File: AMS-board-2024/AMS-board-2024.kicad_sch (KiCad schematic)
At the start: 1 part, among them J1 5077CR-16-SMC2-BK-TR

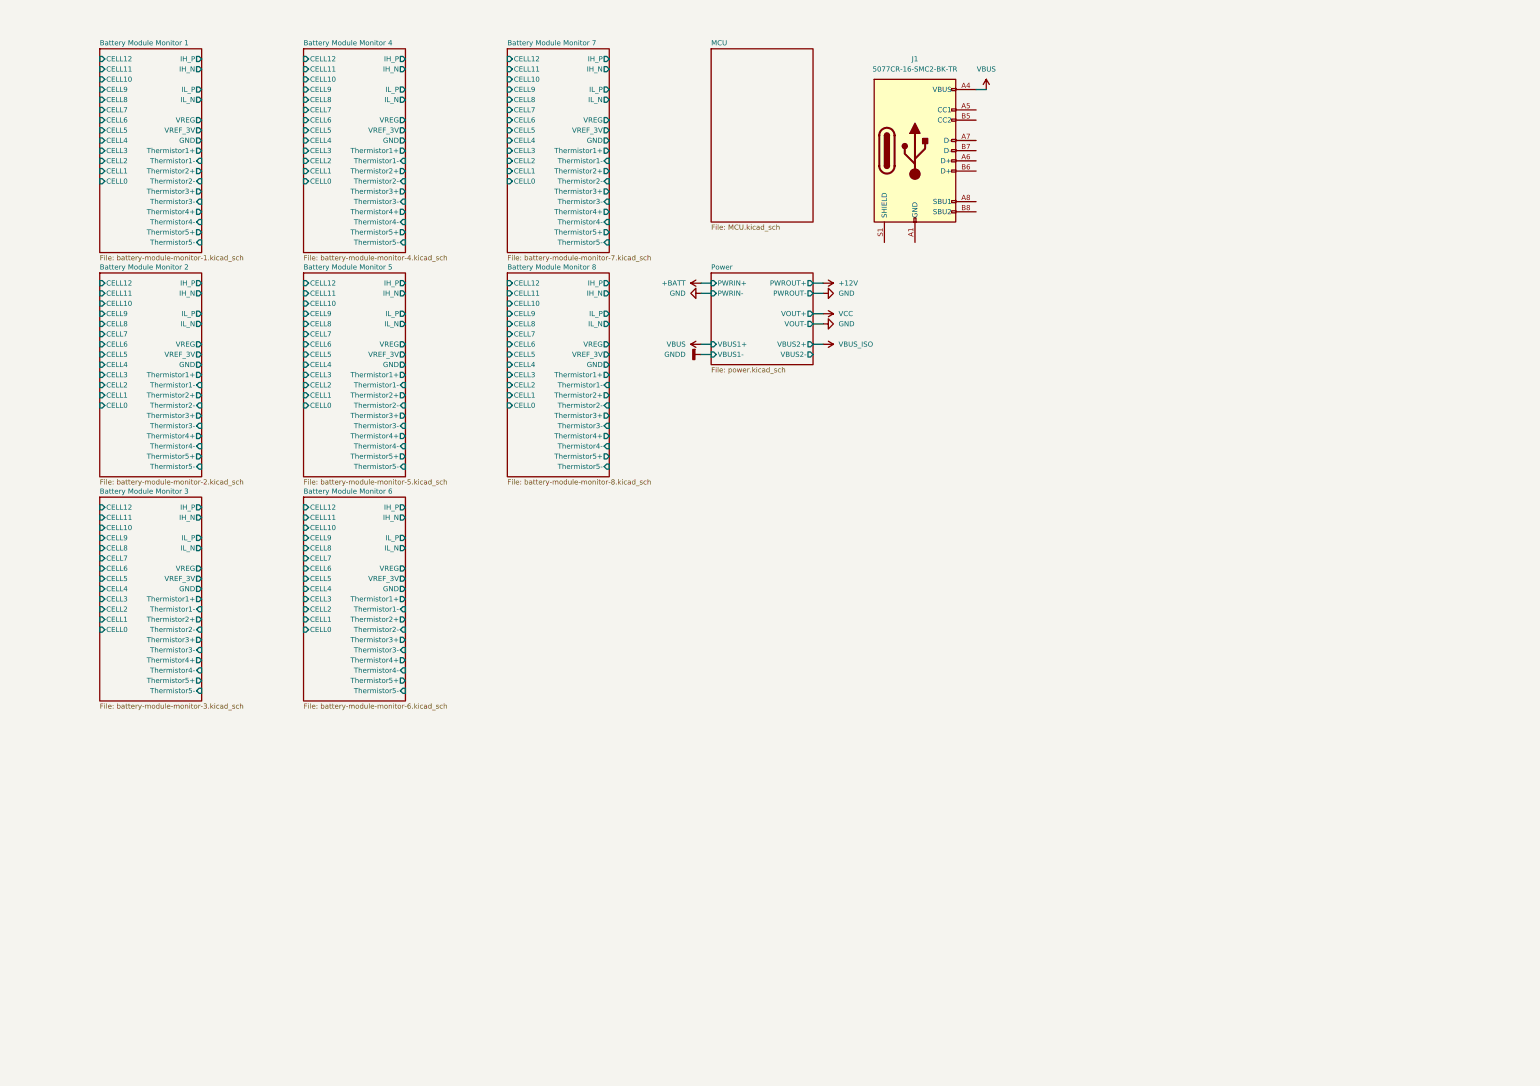
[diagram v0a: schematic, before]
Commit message: アノテーションし直し
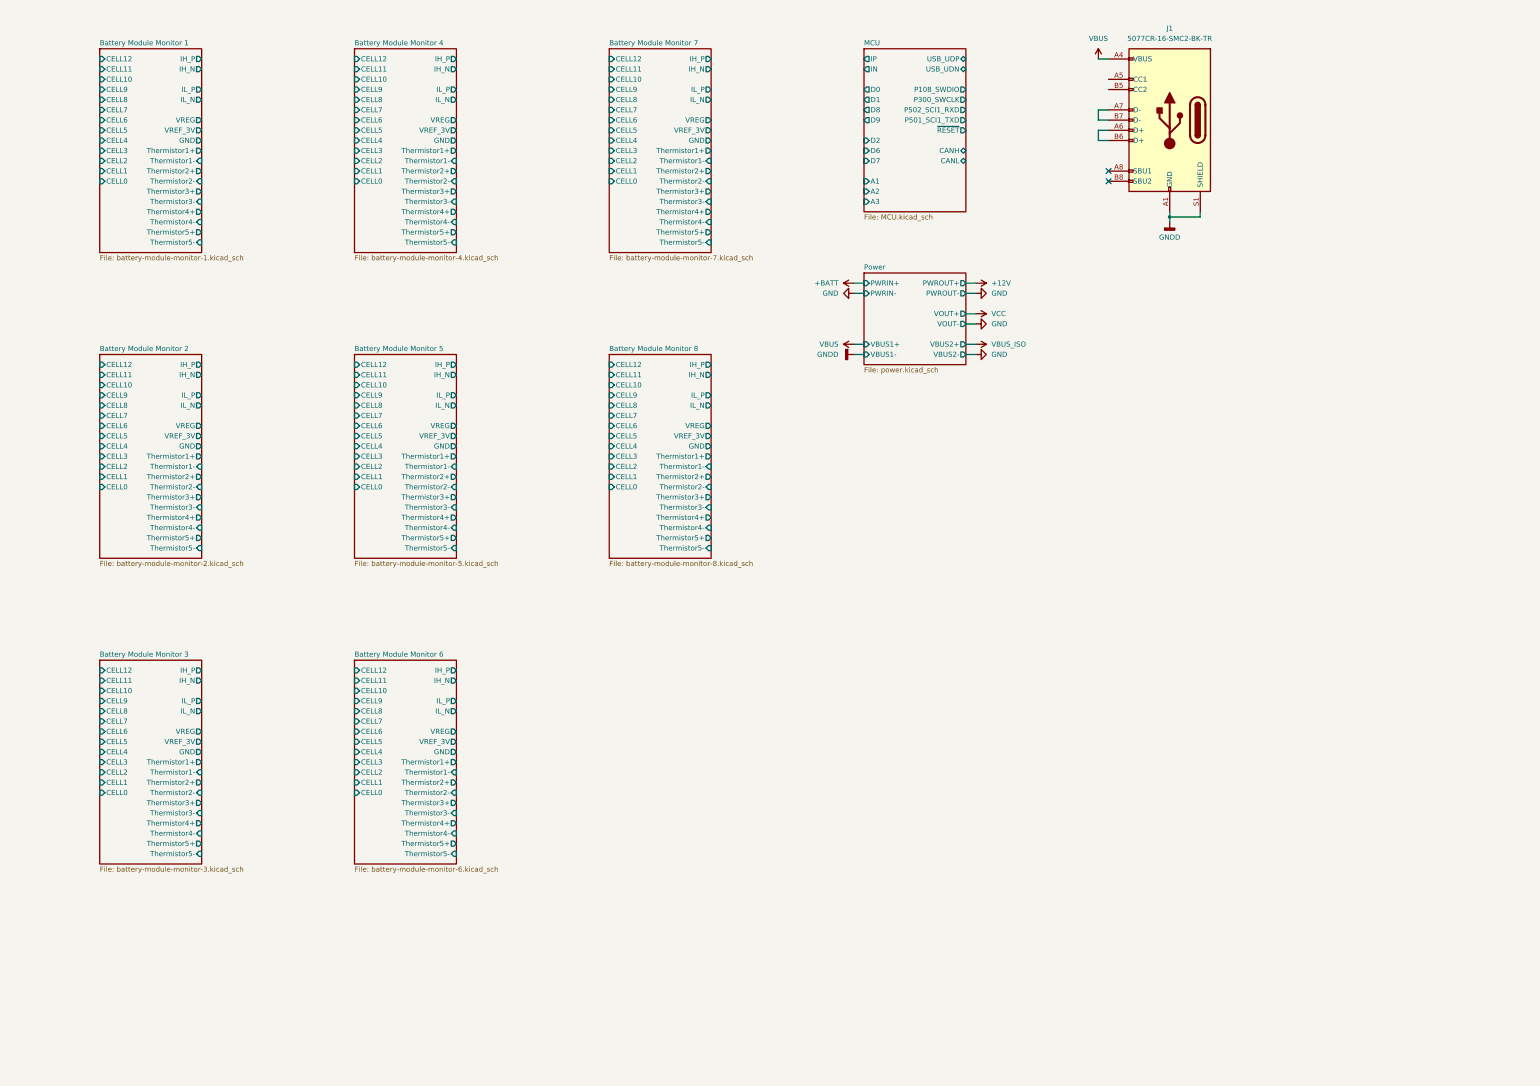
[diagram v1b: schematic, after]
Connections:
- net GNDD: now also J1.A1 (GND), J1.A12 (GND), J1.B1 (GND), J1.B12 (GND), J1.S1 (SHIELD)
- net at J1.A6 (D+): now also J1.B6 (D+)
- net at J1.A7 (D-): now also J1.B7 (D-)
- no-connect marks 0 -> 2
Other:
- sheet MCU ports: added A1, A2, A3, CANH, CANL, D0, D1, D2, D6, D7, D8, D9, IN, IP, P108_SWDIO, P300_SWCLK, P501_SCI1_TXD, P502_SCI1_RXD, USB_UDN, USB_UDP, ~{RESET}; removed none
- moved on the sheet: J1

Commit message: およそ回路図完成
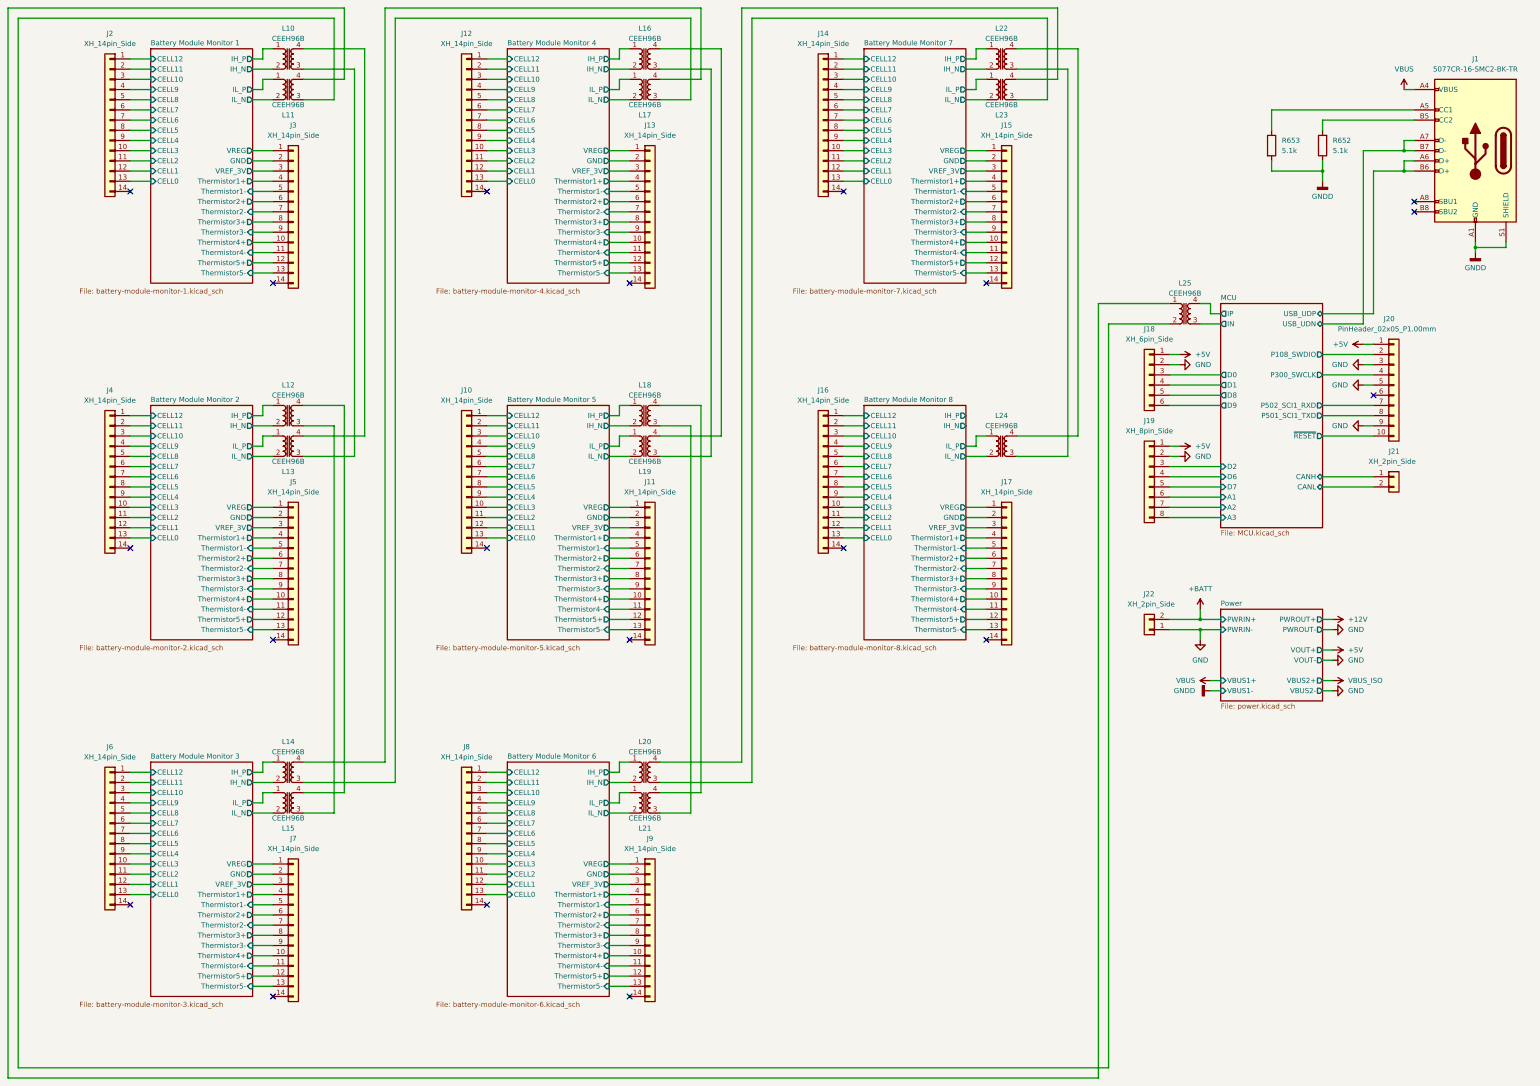
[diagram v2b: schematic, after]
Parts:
- added J10, J11, J12, J13, J14, J15, J16, J17, J2, J3, J4, J5, J6, J7, J8, J9: XH_14pin_Side, Connector_JST:JST_XH_S14B-XH-A_1x14_P2.50mm_Horizontal, symbol Connector_Generic:Conn_01x14
- added J18: XH_6pin_Side, Connector_JST:JST_XH_S6B-XH-A_1x06_P2.50mm_Horizontal, symbol Connector_Generic:Conn_01x06
- added J19: XH_8pin_Side, Connector_JST:JST_XH_S8B-XH-A_1x08_P2.50mm_Horizontal, symbol Connector_Generic:Conn_01x08
- added J20: PinHeader_02x05_P1.00mm, Connector_PinHeader_1.00mm:PinHeader_2x05_P1.00mm_Vertical, symbol Connector_Generic:Conn_01x10
- added J21, J22: XH_2pin_Side, Connector_JST:JST_XH_S2B-XH-A_1x02_P2.50mm_Horizontal, symbol Connector_Generic:Conn_01x02
- added L10, L11, L12, L13, L14, L15, L16, L17, L18, L19, L20, L21, L22, L23, L24, L25: CEEH96B, ProjectEV:Transformer_CEEH96B, symbol ProjectEV:Transfomer_CEEH96B
- added R652, R653: 5.1k, Resistor_SMD:R_0603_1608Metric, symbol Device:R
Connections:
- net +BATT: now also J22.2 (Pin_2)
- net Battery Module Monitor 1/CELL0: now also J2.13 (Pin_13)
- net Battery Module Monitor 1/CELL1: now also J2.12 (Pin_12)
- net Battery Module Monitor 1/CELL10: now also J2.3 (Pin_3)
- net Battery Module Monitor 1/CELL11: now also J2.2 (Pin_2)
- net Battery Module Monitor 1/CELL12: now also J2.1 (Pin_1)
- net Battery Module Monitor 1/CELL2: now also J2.11 (Pin_11)
- net Battery Module Monitor 1/CELL3: now also J2.10 (Pin_10)
- net Battery Module Monitor 1/CELL4: now also J2.9 (Pin_9)
- net Battery Module Monitor 1/CELL5: now also J2.8 (Pin_8)
- net Battery Module Monitor 1/CELL6: now also J2.7 (Pin_7)
- net Battery Module Monitor 1/CELL7: now also J2.6 (Pin_6)
- net Battery Module Monitor 1/CELL8: now also J2.5 (Pin_5)
- net Battery Module Monitor 1/CELL9: now also J2.4 (Pin_4)
- net Battery Module Monitor 1/GND: now also J3.2 (Pin_2)
- net Battery Module Monitor 1/IH_N: now also L10.2
- net Battery Module Monitor 1/IH_P: now also L10.1
- net Battery Module Monitor 1/IL_N: now also L11.2
- net Battery Module Monitor 1/IL_P: now also L11.1
- net Battery Module Monitor 1/Thermistor1+: now also J3.4 (Pin_4)
- net Battery Module Monitor 1/Thermistor1-: now also J3.5 (Pin_5)
- net Battery Module Monitor 1/Thermistor2+: now also J3.6 (Pin_6)
- net Battery Module Monitor 1/Thermistor2-: now also J3.7 (Pin_7)
- net Battery Module Monitor 1/Thermistor3+: now also J3.8 (Pin_8)
- net Battery Module Monitor 1/Thermistor3-: now also J3.9 (Pin_9)
- net Battery Module Monitor 1/Thermistor4+: now also J3.10 (Pin_10)
- net Battery Module Monitor 1/Thermistor4-: now also J3.11 (Pin_11)
- net Battery Module Monitor 1/Thermistor5+: now also J3.12 (Pin_12)
- net Battery Module Monitor 1/Thermistor5-: now also J3.13 (Pin_13)
- net Battery Module Monitor 1/VREF_3V: now also J3.3 (Pin_3)
- net Battery Module Monitor 1/VREG: now also J3.1 (Pin_1)
- net Battery Module Monitor 2/CELL0: now also J4.13 (Pin_13)
- net Battery Module Monitor 2/CELL1: now also J4.12 (Pin_12)
- net Battery Module Monitor 2/CELL10: now also J4.3 (Pin_3)
- net Battery Module Monitor 2/CELL11: now also J4.2 (Pin_2)
- net Battery Module Monitor 2/CELL12: now also J4.1 (Pin_1)
- net Battery Module Monitor 2/CELL2: now also J4.11 (Pin_11)
- net Battery Module Monitor 2/CELL3: now also J4.10 (Pin_10)
- net Battery Module Monitor 2/CELL4: now also J4.9 (Pin_9)
- net Battery Module Monitor 2/CELL5: now also J4.8 (Pin_8)
- net Battery Module Monitor 2/CELL6: now also J4.7 (Pin_7)
- net Battery Module Monitor 2/CELL7: now also J4.6 (Pin_6)
- net Battery Module Monitor 2/CELL8: now also J4.5 (Pin_5)
- net Battery Module Monitor 2/CELL9: now also J4.4 (Pin_4)
- net Battery Module Monitor 2/GND: now also J5.2 (Pin_2)
- net Battery Module Monitor 2/IH_N: now also L12.2
- net Battery Module Monitor 2/IH_P: now also L12.1
- net Battery Module Monitor 2/IL_N: now also L13.2
- net Battery Module Monitor 2/IL_P: now also L13.1
- net Battery Module Monitor 2/Thermistor1+: now also J5.4 (Pin_4)
- net Battery Module Monitor 2/Thermistor1-: now also J5.5 (Pin_5)
- net Battery Module Monitor 2/Thermistor2+: now also J5.6 (Pin_6)
- net Battery Module Monitor 2/Thermistor2-: now also J5.7 (Pin_7)
- net Battery Module Monitor 2/Thermistor3+: now also J5.8 (Pin_8)
- net Battery Module Monitor 2/Thermistor3-: now also J5.9 (Pin_9)
- net Battery Module Monitor 2/Thermistor4+: now also J5.10 (Pin_10)
- net Battery Module Monitor 2/Thermistor4-: now also J5.11 (Pin_11)
- net Battery Module Monitor 2/Thermistor5+: now also J5.12 (Pin_12)
- net Battery Module Monitor 2/Thermistor5-: now also J5.13 (Pin_13)
- net Battery Module Monitor 2/VREF_3V: now also J5.3 (Pin_3)
- net Battery Module Monitor 2/VREG: now also J5.1 (Pin_1)
- net Battery Module Monitor 3/CELL0: now also J6.13 (Pin_13)
- net Battery Module Monitor 3/CELL1: now also J6.12 (Pin_12)
- net Battery Module Monitor 3/CELL10: now also J6.3 (Pin_3)
- net Battery Module Monitor 3/CELL11: now also J6.2 (Pin_2)
- net Battery Module Monitor 3/CELL12: now also J6.1 (Pin_1)
- net Battery Module Monitor 3/CELL2: now also J6.11 (Pin_11)
- net Battery Module Monitor 3/CELL3: now also J6.10 (Pin_10)
- net Battery Module Monitor 3/CELL4: now also J6.9 (Pin_9)
- net Battery Module Monitor 3/CELL5: now also J6.8 (Pin_8)
- net Battery Module Monitor 3/CELL6: now also J6.7 (Pin_7)
- net Battery Module Monitor 3/CELL7: now also J6.6 (Pin_6)
- net Battery Module Monitor 3/CELL8: now also J6.5 (Pin_5)
- net Battery Module Monitor 3/CELL9: now also J6.4 (Pin_4)
- net Battery Module Monitor 3/GND: now also J7.2 (Pin_2)
- net Battery Module Monitor 3/IH_N: now also L14.2
- net Battery Module Monitor 3/IH_P: now also L14.1
- net Battery Module Monitor 3/IL_N: now also L15.2
- net Battery Module Monitor 3/IL_P: now also L15.1
- net Battery Module Monitor 3/Thermistor1+: now also J7.4 (Pin_4)
- net Battery Module Monitor 3/Thermistor1-: now also J7.5 (Pin_5)
- net Battery Module Monitor 3/Thermistor2+: now also J7.6 (Pin_6)
- net Battery Module Monitor 3/Thermistor2-: now also J7.7 (Pin_7)
- net Battery Module Monitor 3/Thermistor3+: now also J7.8 (Pin_8)
- net Battery Module Monitor 3/Thermistor3-: now also J7.9 (Pin_9)
- net Battery Module Monitor 3/Thermistor4+: now also J7.10 (Pin_10)
- net Battery Module Monitor 3/Thermistor4-: now also J7.11 (Pin_11)
- net Battery Module Monitor 3/Thermistor5+: now also J7.12 (Pin_12)
- net Battery Module Monitor 3/Thermistor5-: now also J7.13 (Pin_13)
- net Battery Module Monitor 3/VREF_3V: now also J7.3 (Pin_3)
- net Battery Module Monitor 3/VREG: now also J7.1 (Pin_1)
- net Battery Module Monitor 4/CELL0: now also J12.13 (Pin_13)
- net Battery Module Monitor 4/CELL1: now also J12.12 (Pin_12)
- net Battery Module Monitor 4/CELL10: now also J12.3 (Pin_3)
- net Battery Module Monitor 4/CELL11: now also J12.2 (Pin_2)
- net Battery Module Monitor 4/CELL12: now also J12.1 (Pin_1)
- net Battery Module Monitor 4/CELL2: now also J12.11 (Pin_11)
- net Battery Module Monitor 4/CELL3: now also J12.10 (Pin_10)
- net Battery Module Monitor 4/CELL4: now also J12.9 (Pin_9)
- net Battery Module Monitor 4/CELL5: now also J12.8 (Pin_8)
- net Battery Module Monitor 4/CELL6: now also J12.7 (Pin_7)
- net Battery Module Monitor 4/CELL7: now also J12.6 (Pin_6)
- net Battery Module Monitor 4/CELL8: now also J12.5 (Pin_5)
- net Battery Module Monitor 4/CELL9: now also J12.4 (Pin_4)
- net Battery Module Monitor 4/GND: now also J13.2 (Pin_2)
- net Battery Module Monitor 4/IH_N: now also L16.2
- net Battery Module Monitor 4/IH_P: now also L16.1
- net Battery Module Monitor 4/IL_N: now also L17.2
- net Battery Module Monitor 4/IL_P: now also L17.1
- net Battery Module Monitor 4/Thermistor1+: now also J13.4 (Pin_4)
- net Battery Module Monitor 4/Thermistor1-: now also J13.5 (Pin_5)
- net Battery Module Monitor 4/Thermistor2+: now also J13.6 (Pin_6)
- net Battery Module Monitor 4/Thermistor2-: now also J13.7 (Pin_7)
- net Battery Module Monitor 4/Thermistor3+: now also J13.8 (Pin_8)
- net Battery Module Monitor 4/Thermistor3-: now also J13.9 (Pin_9)
- net Battery Module Monitor 4/Thermistor4+: now also J13.10 (Pin_10)
- net Battery Module Monitor 4/Thermistor4-: now also J13.11 (Pin_11)
- net Battery Module Monitor 4/Thermistor5+: now also J13.12 (Pin_12)
- net Battery Module Monitor 4/Thermistor5-: now also J13.13 (Pin_13)
- net Battery Module Monitor 4/VREF_3V: now also J13.3 (Pin_3)
- net Battery Module Monitor 4/VREG: now also J13.1 (Pin_1)
- net Battery Module Monitor 5/CELL0: now also J10.13 (Pin_13)
- net Battery Module Monitor 5/CELL1: now also J10.12 (Pin_12)
- net Battery Module Monitor 5/CELL10: now also J10.3 (Pin_3)
- net Battery Module Monitor 5/CELL11: now also J10.2 (Pin_2)
- net Battery Module Monitor 5/CELL12: now also J10.1 (Pin_1)
- net Battery Module Monitor 5/CELL2: now also J10.11 (Pin_11)
- net Battery Module Monitor 5/CELL3: now also J10.10 (Pin_10)
- net Battery Module Monitor 5/CELL4: now also J10.9 (Pin_9)
- net Battery Module Monitor 5/CELL5: now also J10.8 (Pin_8)
- net Battery Module Monitor 5/CELL6: now also J10.7 (Pin_7)
- net Battery Module Monitor 5/CELL7: now also J10.6 (Pin_6)
- net Battery Module Monitor 5/CELL8: now also J10.5 (Pin_5)
- net Battery Module Monitor 5/CELL9: now also J10.4 (Pin_4)
- net Battery Module Monitor 5/GND: now also J11.2 (Pin_2)
- net Battery Module Monitor 5/IH_N: now also L18.2
- net Battery Module Monitor 5/IH_P: now also L18.1
- net Battery Module Monitor 5/IL_N: now also L19.2
- net Battery Module Monitor 5/IL_P: now also L19.1
- net Battery Module Monitor 5/Thermistor1+: now also J11.4 (Pin_4)
- net Battery Module Monitor 5/Thermistor1-: now also J11.5 (Pin_5)
- net Battery Module Monitor 5/Thermistor2+: now also J11.6 (Pin_6)
- net Battery Module Monitor 5/Thermistor2-: now also J11.7 (Pin_7)
- net Battery Module Monitor 5/Thermistor3+: now also J11.8 (Pin_8)
- net Battery Module Monitor 5/Thermistor3-: now also J11.9 (Pin_9)
- net Battery Module Monitor 5/Thermistor4+: now also J11.10 (Pin_10)
- net Battery Module Monitor 5/Thermistor4-: now also J11.11 (Pin_11)
- net Battery Module Monitor 5/Thermistor5+: now also J11.12 (Pin_12)
- net Battery Module Monitor 5/Thermistor5-: now also J11.13 (Pin_13)
- net Battery Module Monitor 5/VREF_3V: now also J11.3 (Pin_3)
- net Battery Module Monitor 5/VREG: now also J11.1 (Pin_1)
- net Battery Module Monitor 6/CELL0: now also J8.13 (Pin_13)
- net Battery Module Monitor 6/CELL1: now also J8.12 (Pin_12)
- net Battery Module Monitor 6/CELL10: now also J8.3 (Pin_3)
- net Battery Module Monitor 6/CELL11: now also J8.2 (Pin_2)
- net Battery Module Monitor 6/CELL12: now also J8.1 (Pin_1)
- net Battery Module Monitor 6/CELL2: now also J8.11 (Pin_11)
- net Battery Module Monitor 6/CELL3: now also J8.10 (Pin_10)
- net Battery Module Monitor 6/CELL4: now also J8.9 (Pin_9)
- net Battery Module Monitor 6/CELL5: now also J8.8 (Pin_8)
- net Battery Module Monitor 6/CELL6: now also J8.7 (Pin_7)
- net Battery Module Monitor 6/CELL7: now also J8.6 (Pin_6)
- net Battery Module Monitor 6/CELL8: now also J8.5 (Pin_5)
- net Battery Module Monitor 6/CELL9: now also J8.4 (Pin_4)
- net Battery Module Monitor 6/GND: now also J9.2 (Pin_2)
- net Battery Module Monitor 6/IH_N: now also L20.2
- net Battery Module Monitor 6/IH_P: now also L20.1
- net Battery Module Monitor 6/IL_N: now also L21.2
- net Battery Module Monitor 6/IL_P: now also L21.1
- net Battery Module Monitor 6/Thermistor1+: now also J9.4 (Pin_4)
- net Battery Module Monitor 6/Thermistor1-: now also J9.5 (Pin_5)
- net Battery Module Monitor 6/Thermistor2+: now also J9.6 (Pin_6)
- net Battery Module Monitor 6/Thermistor2-: now also J9.7 (Pin_7)
- net Battery Module Monitor 6/Thermistor3+: now also J9.8 (Pin_8)
- net Battery Module Monitor 6/Thermistor3-: now also J9.9 (Pin_9)
- net Battery Module Monitor 6/Thermistor4+: now also J9.10 (Pin_10)
- net Battery Module Monitor 6/Thermistor4-: now also J9.11 (Pin_11)
- net Battery Module Monitor 6/Thermistor5+: now also J9.12 (Pin_12)
- net Battery Module Monitor 6/Thermistor5-: now also J9.13 (Pin_13)
- net Battery Module Monitor 6/VREF_3V: now also J9.3 (Pin_3)
- net Battery Module Monitor 6/VREG: now also J9.1 (Pin_1)
- net Battery Module Monitor 7/CELL0: now also J14.13 (Pin_13)
- net Battery Module Monitor 7/CELL1: now also J14.12 (Pin_12)
- net Battery Module Monitor 7/CELL10: now also J14.3 (Pin_3)
- net Battery Module Monitor 7/CELL11: now also J14.2 (Pin_2)
- net Battery Module Monitor 7/CELL12: now also J14.1 (Pin_1)
- net Battery Module Monitor 7/CELL2: now also J14.11 (Pin_11)
- net Battery Module Monitor 7/CELL3: now also J14.10 (Pin_10)
- net Battery Module Monitor 7/CELL4: now also J14.9 (Pin_9)
- net Battery Module Monitor 7/CELL5: now also J14.8 (Pin_8)
- net Battery Module Monitor 7/CELL6: now also J14.7 (Pin_7)
- net Battery Module Monitor 7/CELL7: now also J14.6 (Pin_6)
- net Battery Module Monitor 7/CELL8: now also J14.5 (Pin_5)
- net Battery Module Monitor 7/CELL9: now also J14.4 (Pin_4)
- net Battery Module Monitor 7/GND: now also J15.2 (Pin_2)
- net Battery Module Monitor 7/IH_N: now also L22.2
- net Battery Module Monitor 7/IH_P: now also L22.1
- net Battery Module Monitor 7/IL_N: now also L23.2
- net Battery Module Monitor 7/IL_P: now also L23.1
- net Battery Module Monitor 7/Thermistor1+: now also J15.4 (Pin_4)
- net Battery Module Monitor 7/Thermistor1-: now also J15.5 (Pin_5)
- net Battery Module Monitor 7/Thermistor2+: now also J15.6 (Pin_6)
- net Battery Module Monitor 7/Thermistor2-: now also J15.7 (Pin_7)
- net Battery Module Monitor 7/Thermistor3+: now also J15.8 (Pin_8)
- net Battery Module Monitor 7/Thermistor3-: now also J15.9 (Pin_9)
- net Battery Module Monitor 7/Thermistor4+: now also J15.10 (Pin_10)
- net Battery Module Monitor 7/Thermistor4-: now also J15.11 (Pin_11)
- net Battery Module Monitor 7/Thermistor5+: now also J15.12 (Pin_12)
- net Battery Module Monitor 7/Thermistor5-: now also J15.13 (Pin_13)
- net Battery Module Monitor 7/VREF_3V: now also J15.3 (Pin_3)
- net Battery Module Monitor 7/VREG: now also J15.1 (Pin_1)
- net Battery Module Monitor 8/CELL0: now also J16.13 (Pin_13)
- net Battery Module Monitor 8/CELL1: now also J16.12 (Pin_12)
- net Battery Module Monitor 8/CELL10: now also J16.3 (Pin_3)
- net Battery Module Monitor 8/CELL11: now also J16.2 (Pin_2)
- net Battery Module Monitor 8/CELL12: now also J16.1 (Pin_1)
- net Battery Module Monitor 8/CELL2: now also J16.11 (Pin_11)
- net Battery Module Monitor 8/CELL3: now also J16.10 (Pin_10)
- net Battery Module Monitor 8/CELL4: now also J16.9 (Pin_9)
- net Battery Module Monitor 8/CELL5: now also J16.8 (Pin_8)
- net Battery Module Monitor 8/CELL6: now also J16.7 (Pin_7)
- net Battery Module Monitor 8/CELL7: now also J16.6 (Pin_6)
- net Battery Module Monitor 8/CELL8: now also J16.5 (Pin_5)
- net Battery Module Monitor 8/CELL9: now also J16.4 (Pin_4)
- net Battery Module Monitor 8/GND: now also J17.2 (Pin_2)
- net Battery Module Monitor 8/IL_N: now also L24.2
- net Battery Module Monitor 8/IL_P: now also L24.1
- net Battery Module Monitor 8/Thermistor1+: now also J17.4 (Pin_4)
- net Battery Module Monitor 8/Thermistor1-: now also J17.5 (Pin_5)
- net Battery Module Monitor 8/Thermistor2+: now also J17.6 (Pin_6)
- net Battery Module Monitor 8/Thermistor2-: now also J17.7 (Pin_7)
- net Battery Module Monitor 8/Thermistor3+: now also J17.8 (Pin_8)
- net Battery Module Monitor 8/Thermistor3-: now also J17.9 (Pin_9)
- net Battery Module Monitor 8/Thermistor4+: now also J17.10 (Pin_10)
- net Battery Module Monitor 8/Thermistor4-: now also J17.11 (Pin_11)
- net Battery Module Monitor 8/Thermistor5+: now also J17.12 (Pin_12)
- net Battery Module Monitor 8/Thermistor5-: now also J17.13 (Pin_13)
- net Battery Module Monitor 8/VREF_3V: now also J17.3 (Pin_3)
- net Battery Module Monitor 8/VREG: now also J17.1 (Pin_1)
- net GND: now also J18.2 (Pin_2), J19.2 (Pin_2), J20.3 (Pin_3), J20.5 (Pin_5), J20.9 (Pin_9), J22.1 (Pin_1)
- net GNDD: now also R652.1, R653.2
- net MCU/A1: now also J19.6 (Pin_6)
- net MCU/A2: now also J19.7 (Pin_7)
- net MCU/A3: now also J19.8 (Pin_8)
- net MCU/CANH: now also J21.1 (Pin_1)
- net MCU/CANL: now also J21.2 (Pin_2)
- net MCU/D0: now also J18.3 (Pin_3)
- net MCU/D1: now also J18.4 (Pin_4)
- net MCU/D2: now also J19.3 (Pin_3)
- net MCU/D6: now also J19.4 (Pin_4)
- net MCU/D7: now also J19.5 (Pin_5)
- net MCU/D8: now also J18.5 (Pin_5)
- net MCU/D9: now also J18.6 (Pin_6)
- net MCU/IN: now also L25.3
- net MCU/IP: now also L25.4
- net MCU/P108_SWDIO: now also J20.2 (Pin_2)
- net MCU/P300_SWCLK: now also J20.4 (Pin_4)
- net MCU/P501_SCI1_TXD: now also J20.8 (Pin_8)
- net MCU/P502_SCI1_RXD: now also J20.7 (Pin_7)
- net MCU/USB_UDN: now also J1.A7 (D-), J1.B7 (D-)
- net MCU/USB_UDP: now also J1.A6 (D+), J1.B6 (D+)
- net MCU/~{RESET}: now also J20.10 (Pin_10)
- net at J1.A5 (CC1): now also R653.1
- net at J1.B5 (CC2): now also R652.2
- new net: L16.3, L19.3
- new net: L16.4, L19.4
- new net: L18.3, L21.3
- new net: L18.4, L21.4
- new net: L11.3, L25.2
- new net: L11.4, L25.1
- new net: L12.3, L15.3
- new net: L12.4, L15.4
- new net: L14.3, L17.3
- new net: L14.4, L17.4
- new net: L22.3, L24.3
- new net: L22.4, L24.4
- new net: L10.3, L13.3
- new net: L10.4, L13.4
- new net: L20.3, L23.3
- new net: L20.4, L23.4
- new net +5V: J18.1 (Pin_1), J19.1 (Pin_1), J20.1 (Pin_1)
- no-connect marks 2 -> 19
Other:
- moved on the sheet: J1
